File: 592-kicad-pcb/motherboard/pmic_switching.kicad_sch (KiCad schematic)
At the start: 5 parts

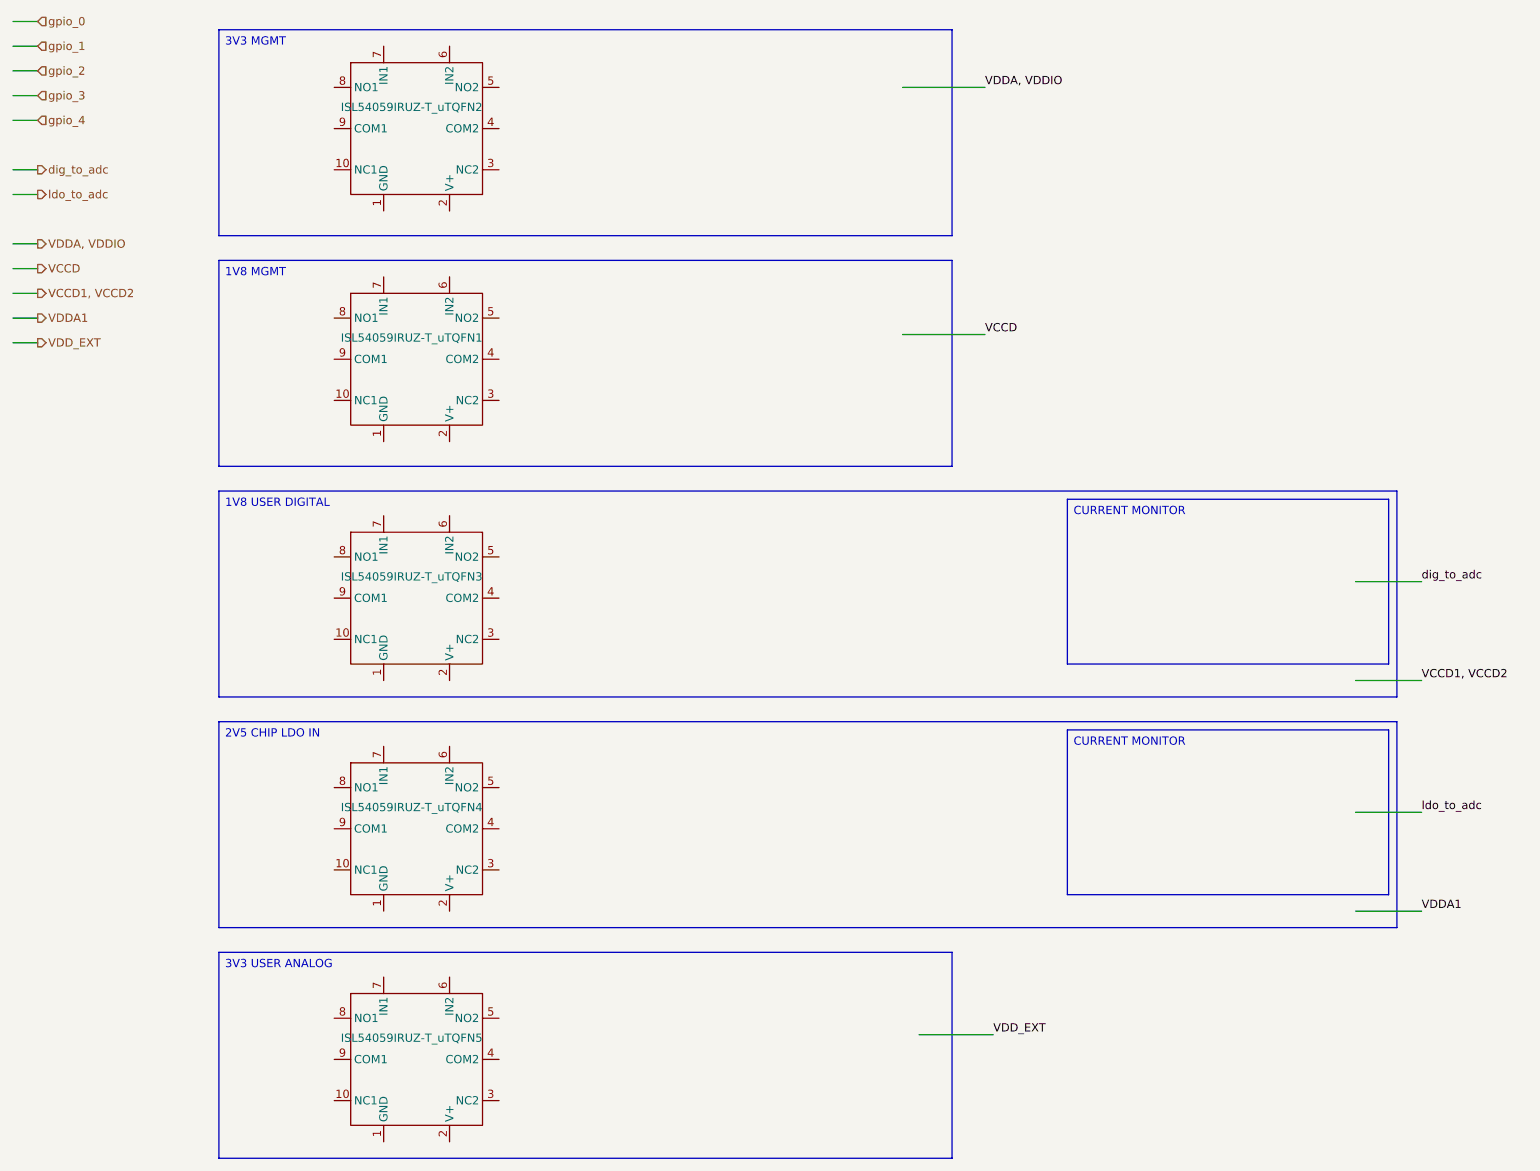
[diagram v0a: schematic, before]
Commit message: current monitor symbol
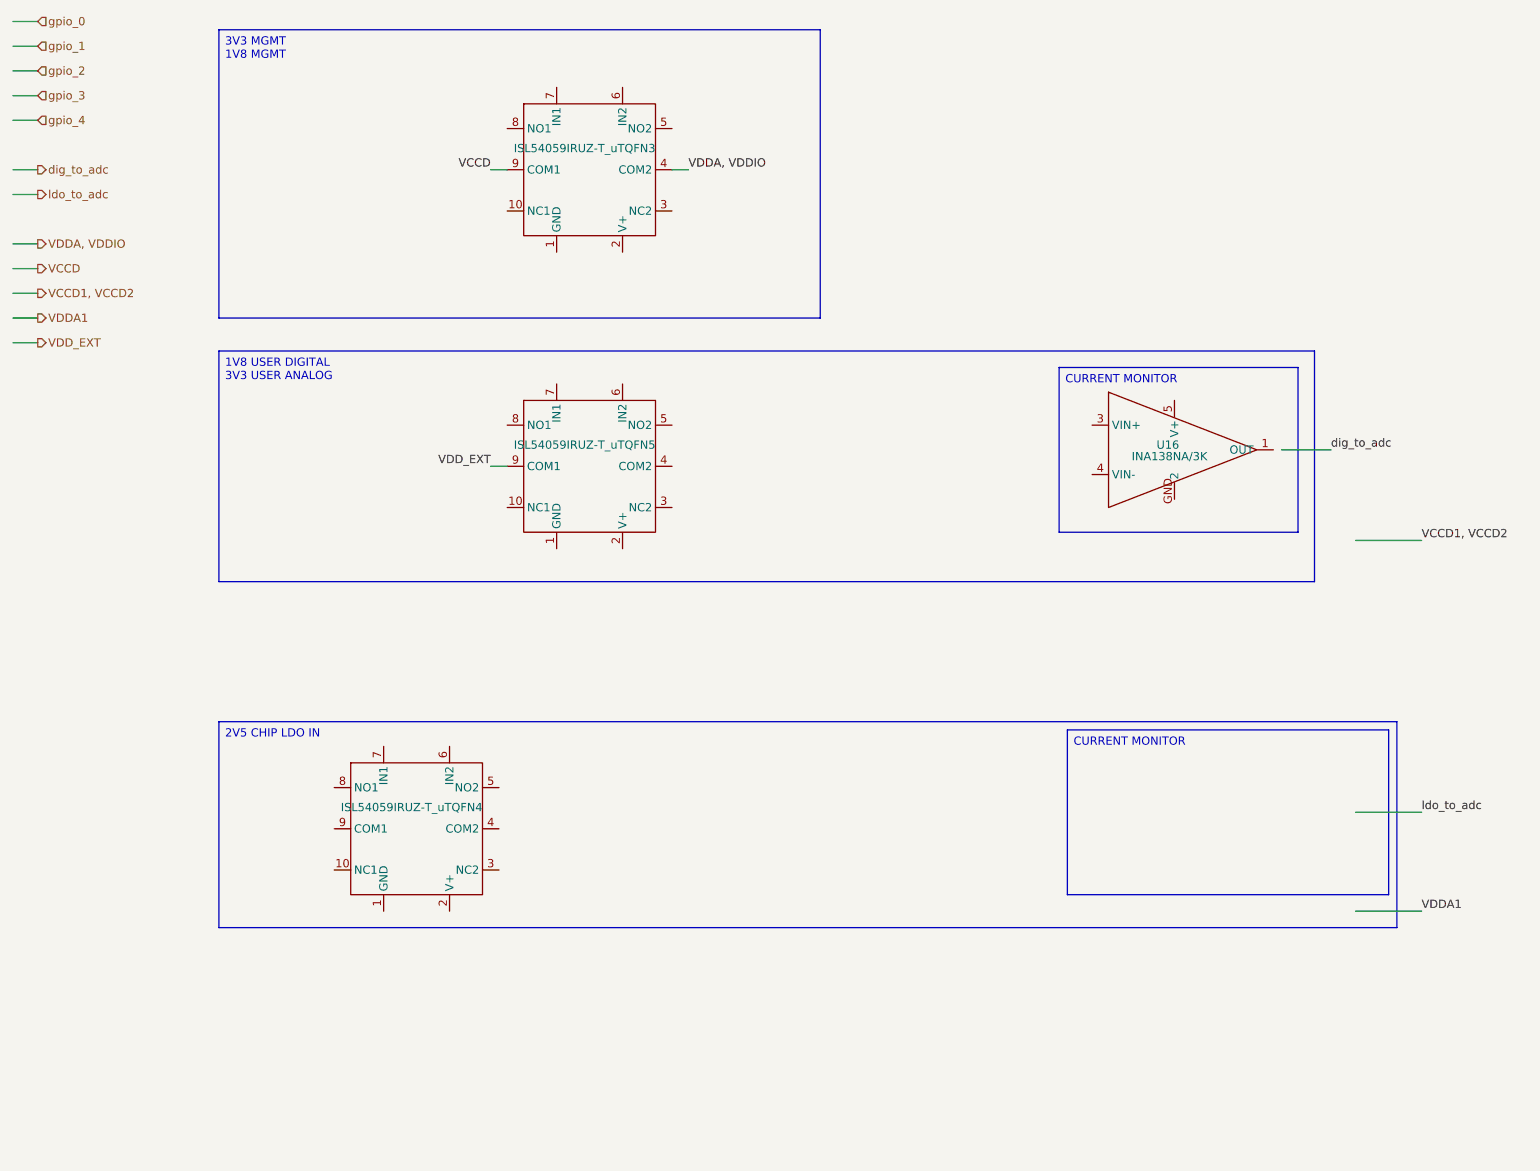
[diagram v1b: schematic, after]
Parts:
- removed ISL54059IRUZ-T_uTQFN1, ISL54059IRUZ-T_uTQFN2: ~, symbol 592-partslib:ISL54059IRUZ-T_uTQFN
- added U16: INA138NA/3K, symbol 592-partslib:INA138NA/3K
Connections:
- net VCCD: now also ISL54059IRUZ-T_uTQFN3.9 (COM1)
- net VDDA, VDDIO: now also ISL54059IRUZ-T_uTQFN3.4 (COM2)
- net VDD_EXT: now also ISL54059IRUZ-T_uTQFN5.9 (COM1)
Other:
- moved on the sheet: ISL54059IRUZ-T_uTQFN3, ISL54059IRUZ-T_uTQFN5
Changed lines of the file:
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@@
 		(rev "0.00")
 	)
-	(text_box "1V8 USER DIGITAL"
-		(exclude_from_sim no)
-		(at 46.99 87.63 0)
-		(size 181.61 31.75)
+	(text_box "1V8 USER DIGITAL\n3V3 USER ANALOG"
+		(exclude_from_sim no)
+		(at 46.99 66.04 0)
+		(size 168.91 35.56)
 		(margins 0.9525 0.9525 0.9525 0.9525)
 		(stroke
@@
 		)
 	)
-	(text_box "3V3 USER ANALOG"
-		(exclude_from_sim no)
-		(at 46.99 158.75 0)
-		(size 113.03 31.75)
+	(text_box "3V3 MGMT\n1V8 MGMT"
+		(exclude_from_sim no)
+		(at 46.99 16.51 0)
+		(size 92.71 44.45)
 		(margins 0.9525 0.9525 0.9525 0.9525)
 		(stroke
@@
 		)
 	)
-	(text_box "3V3 MGMT"
-		(exclude_from_sim no)
-		(at 46.99 16.51 0)
-		(size 113.03 31.75)
-		(margins 0.9525 0.9525 0.9525 0.9525)
-		(stroke
-			(width 0)
-			(type solid)
-		)
-		(fill
-			(type none)
-		)
-		(effects
-			(font
-				(size 1.27 1.27)
-			)
-			(justify left top)
-		)
-	)
 	(text_box "CURRENT MONITOR"
 		(exclude_from_sim no)
-		(at 177.8 88.9 0)
-		(size 49.53 25.4)
+		(at 176.53 68.58 0)
+		(size 36.83 25.4)
 		(margins 0.9525 0.9525 0.9525 0.9525)
 		(stroke
@@
 		)
 	)
-	(text_box "1V8 MGMT"
-		(exclude_from_sim no)
-		(at 46.99 52.07 0)
-		(size 113.03 31.75)
-		(margins 0.9525 0.9525 0.9525 0.9525)
-		(stroke
-			(width 0)
-			(type solid)
-		)
-		(fill
-			(type none)
-		)
-		(effects
-			(font
-				(size 1.27 1.27)
-			)
-			(justify left top)
-		)
-	)
 	(wire
 		(pts
@@
 	(wire
 		(pts
-			(xy 152.4 63.5) (xy 165.1 63.5)
+			(xy 91.44 38.1) (xy 88.9 38.1)
 		)
 		(stroke
@@
 	(wire
 		(pts
-			(xy 222.25 101.6) (xy 232.41 101.6)
+			(xy 210.82 81.28) (xy 218.44 81.28)
 		)
 		(stroke
@@
 	(wire
 		(pts
-			(xy 152.4 25.4) (xy 165.1 25.4)
+			(xy 116.84 38.1) (xy 119.38 38.1)
 		)
 		(stroke
@@
 	(wire
 		(pts
-			(xy 222.25 116.84) (xy 232.41 116.84)
+			(xy 222.25 95.25) (xy 232.41 95.25)
 		)
 		(stroke
@@
 	(wire
 		(pts
-			(xy 154.94 171.45) (xy 166.37 171.45)
+			(xy 91.44 83.82) (xy 88.9 83.82)
 		)
 		(stroke
@@
 	)
 	(label "dig_to_adc"
-		(at 232.41 101.6 0)
+		(at 218.44 81.28 0)
 		(effects
 			(font
@@
 	)
 	(label "VCCD"
-		(at 165.1 63.5 0)
+		(at 88.9 38.1 180)
+		(effects
+			(font
+				(size 1.27 1.27)
+			)
+			(justify right bottom)
+		)
+	)
+	(label "VDDA, VDDIO"
+		(at 119.38 38.1 0)
 		(effects
 			(font
@@
 		)
 	)
-	(label "VDDA, VDDIO"
-		(at 165.1 25.4 0)
-		(effects
-			(font
-				(size 1.27 1.27)
-			)
-			(justify left bottom)
-		)
-	)
 	(label "VCCD1, VCCD2"
-		(at 232.41 116.84 0)
+		(at 232.41 95.25 0)
 		(effects
 			(font
@@
 	)
 	(label "VDD_EXT"
-		(at 166.37 171.45 0)
-		(effects
-			(font
-				(size 1.27 1.27)
-			)
-			(justify left bottom)
+		(at 88.9 83.82 180)
+		(effects
+			(font
+				(size 1.27 1.27)
+			)
+			(justify right bottom)
 		)
 	)
@@
 	(symbol
 		(lib_id "592-partslib:ISL54059IRUZ-T_uTQFN")
-		(at 77.47 175.26 0)
+		(at 104.14 83.82 0)
 		(unit 1)
 		(exclude_from_sim no)
@@
 		(dnp no)
 		(property "Reference" "ISL54059IRUZ-T_uTQFN5"
-			(at 65.786 171.958 0)
+			(at 92.456 80.518 0)
 			(effects
 				(font
@@
 		)
 		(property "Value" "~"
-			(at 64.77 171.958 0)
+			(at 91.44 80.518 0)
 			(effects
 				(font
@@
 		)
 		(property "Footprint" ""
-			(at 77.47 175.26 0)
+			(at 104.14 83.82 0)
 			(effects
 				(font
@@
 		)
 		(property "Datasheet" ""
-			(at 77.47 175.26 0)
+			(at 104.14 83.82 0)
 			(effects
 				(font
@@
 		)
 		(property "Description" ""
-			(at 77.47 175.26 0)
+			(at 104.14 83.82 0)
 			(effects
 				(font
@@
 	)
 	(symbol
-		(lib_id "592-partslib:ISL54059IRUZ-T_uTQFN")
-		(at 77.47 67.31 0)
+		(lib_id "592-partslib:INA138NA/3K")
+		(at 193.04 81.28 0)
 		(unit 1)
 		(exclude_from_sim no)
@@
 		(on_board yes)
 		(dnp no)
-		(property "Reference" "ISL54059IRUZ-T_uTQFN1"
-			(at 65.786 64.008 0)
-			(effects
-				(font
-					(size 1.27 1.27)
-				)
-				(justify left)
-			)
-		)
-		(property "Value" "~"
-			(at 64.77 64.008 0)
-			(effects
-				(font
-					(size 1.27 1.27)
-				)
-				(justify left)
+		(property "Reference" "U16"
+			(at 193.294 80.518 0)
+			(effects
+				(font
+					(size 1.27 1.27)
+				)
+			)
+		)
+		(property "Value" "INA138NA/3K"
+			(at 193.548 82.296 0)
+			(effects
+				(font
+					(size 1.27 1.27)
+				)
 			)
 		)
 		(property "Footprint" ""
-			(at 77.47 67.31 0)
-			(effects
-				(font
-					(size 1.27 1.27)
-				)
-				(hide yes)
-			)
-		)
-		(property "Datasheet" ""
-			(at 77.47 67.31 0)
-			(effects
-				(font
-					(size 1.27 1.27)
-				)
-				(hide yes)
-			)
-		)
-		(property "Description" ""
-			(at 77.47 67.31 0)
+			(at 193.04 81.28 0)
+			(effects
+				(font
+					(size 1.27 1.27)
+				)
+				(hide yes)
+			)
+		)
+		(property "Datasheet" "https://www.lcsc.com/datasheet/C47914.pdf"
+			(at 193.04 81.28 0)
+			(effects
+				(font
+					(size 1.27 1.27)
+				)
+				(hide yes)
+			)
+		)
+		(property "Description" "TI current monitor"
+			(at 193.04 81.28 0)
 			(effects
 				(font
@@
 		(pin "5"
 		)
+		(pin "3"
+		)
 		(pin "4"
 		)
-		(pin "8"
-		)
-		(pin "3"
-		)
-		(pin "9"
-		)
-		(pin "7"
-		)
 		(pin "1"
 		)
-		(pin "2"
-		)
-		(pin "6"
-		)
-		(pin "10"
+		(pin "GND"
 		)
 		(instances
 			(project ""
 				(path "/5b0c97ac-fa03-4db8-b41b-0eee32b6f55d/f049e4ad-bebe-4338-850a-2727de737ae9/260af3dc-9286-4c76-9c6c-eeb806d3e6e5"
-					(reference "ISL54059IRUZ-T_uTQFN1")
+					(reference "U16")
 					(unit 1)
 				)
@@
 	(symbol
 		(lib_id "592-partslib:ISL54059IRUZ-T_uTQFN")
-		(at 77.47 31.75 0)
-		(unit 1)
-		(exclude_from_sim no)
-		(in_bom yes)
-		(on_board yes)
-		(dnp no)
-		(property "Reference" "ISL54059IRUZ-T_uTQFN2"
-			(at 65.786 28.448 0)
-			(effects
-				(font
-					(size 1.27 1.27)
-				)
-				(justify left)
-			)
-		)
-		(property "Value" "~"
-			(at 64.77 28.448 0)
-			(effects
-				(font
-					(size 1.27 1.27)
-				)
-				(justify left)
-			)
-		)
-		(property "Footprint" ""
-			(at 77.47 31.75 0)
-			(effects
-				(font
-					(size 1.27 1.27)
-				)
-				(hide yes)
-			)
-		)
-		(property "Datasheet" ""
-			(at 77.47 31.75 0)
-			(effects
-				(font
-					(size 1.27 1.27)
-				)
-				(hide yes)
-			)
-		)
-		(property "Description" ""
-			(at 77.47 31.75 0)
-			(effects
-				(font
-					(size 1.27 1.27)
-				)
-				(hide yes)
-			)
-		)
-		(pin "5"
-		)
-		(pin "4"
-		)
-		(pin "8"
-		)
-		(pin "3"
-		)
-		(pin "9"
-		)
-		(pin "7"
-		)
-		(pin "1"
-		)
-		(pin "2"
-		)
-		(pin "6"
-		)
-		(pin "10"
-		)
-		(instances
-			(project "motherboard"
-				(path "/5b0c97ac-fa03-4db8-b41b-0eee32b6f55d/f049e4ad-bebe-4338-850a-2727de737ae9/260af3dc-9286-4c76-9c6c-eeb806d3e6e5"
-					(reference "ISL54059IRUZ-T_uTQFN2")
-					(unit 1)
-				)
-			)
-		)
-	)
-	(symbol
-		(lib_id "592-partslib:ISL54059IRUZ-T_uTQFN")
-		(at 77.47 104.14 0)
+		(at 104.14 38.1 0)
 		(unit 1)
 		(exclude_from_sim no)
@@
 		(dnp no)
 		(property "Reference" "ISL54059IRUZ-T_uTQFN3"
-			(at 65.786 100.838 0)
+			(at 92.456 34.798 0)
 			(effects
 				(font
@@
 		)
 		(property "Value" "~"
-			(at 64.77 100.838 0)
+			(at 91.44 34.798 0)
 			(effects
 				(font
@@
 		)
 		(property "Footprint" ""
-			(at 77.47 104.14 0)
+			(at 104.14 38.1 0)
 			(effects
 				(font
@@
 		)
 		(property "Datasheet" ""
-			(at 77.47 104.14 0)
+			(at 104.14 38.1 0)
 			(effects
 				(font
@@
 		)
 		(property "Description" ""
-			(at 77.47 104.14 0)
-			(effects
-				(font
+			(at 104.14 38.1 0)
+			(effects
+				(font
